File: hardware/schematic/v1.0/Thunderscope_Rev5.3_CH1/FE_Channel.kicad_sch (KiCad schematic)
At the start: 105 parts, among them J1002_1 BNC, K1000_1 G6K-2F-RF, K1001_1 G6K-2F-RF, Q1002_1 DMN62D0UW, Q1003_1 DMN62D0UW, U1001_1 TMUX4053, U1008_1 LMH6518, U1009_1 BUF802, U1011_1 OPA140AIDBVR

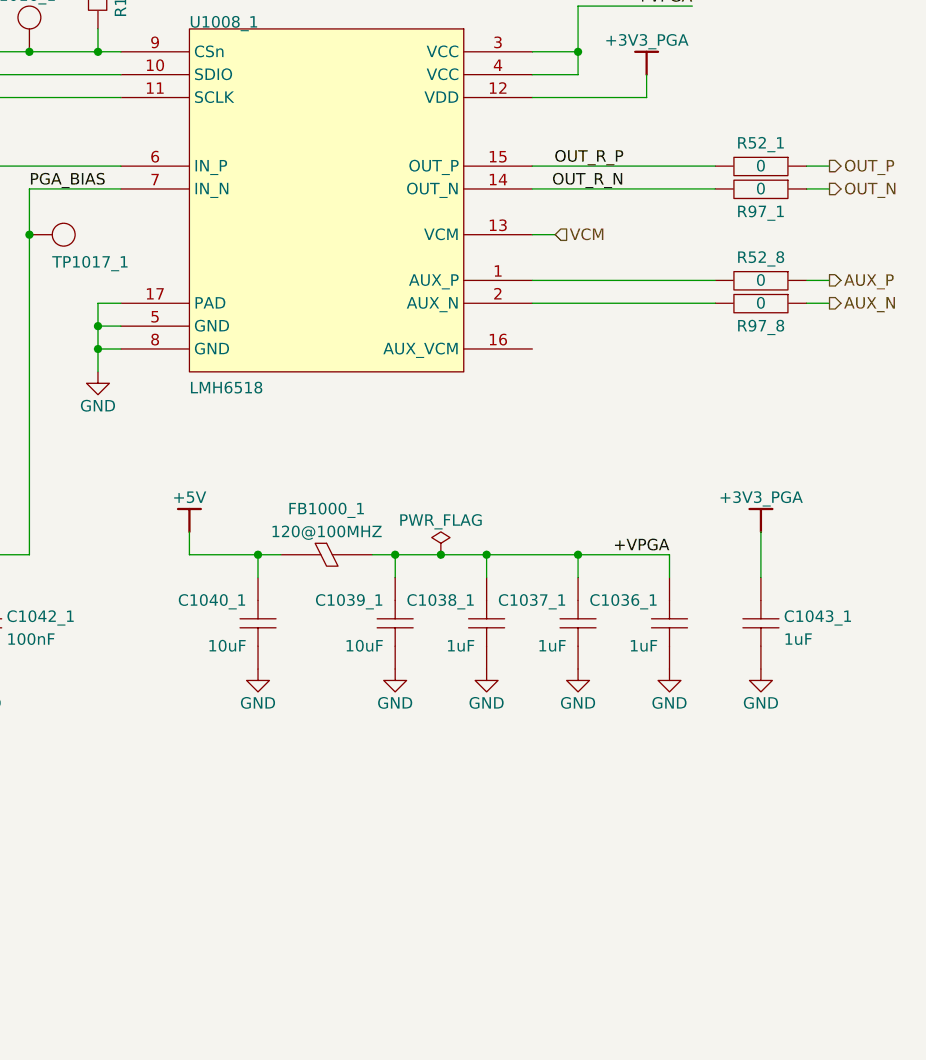
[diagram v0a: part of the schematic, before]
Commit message: sch and pcb update
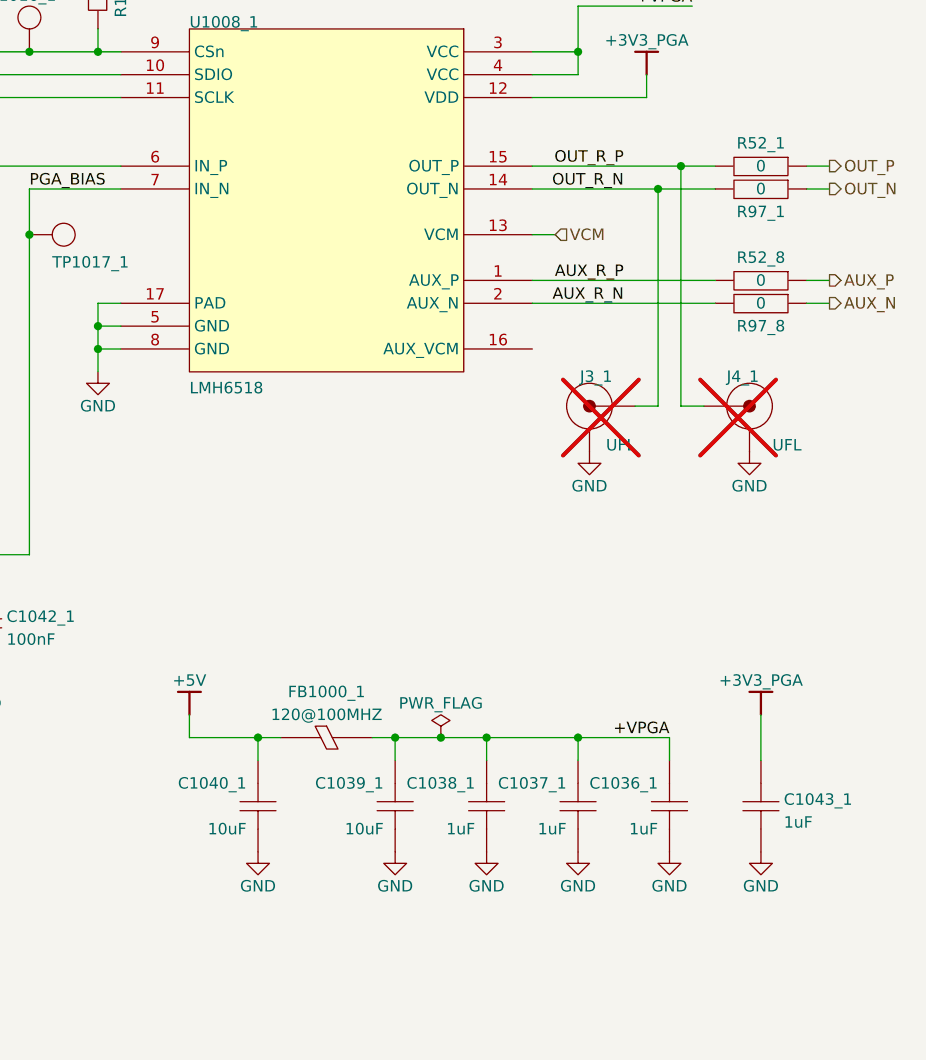
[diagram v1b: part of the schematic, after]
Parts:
- added J3_1, J4_1: UFL, Thunderscope_Rev5:TE_2334884-1, symbol Thunderscope_Rev5:UFL Jack SMD
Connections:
- net GND: now also J3_1.2 (SHIELD), J4_1.2 (SHIELD)
- net OUT_R_N: now also J3_1.1 (Signal)
- net OUT_R_P: now also J4_1.1 (Signal)
- net AUX_R_P: now reaches R52_8.1, U1008_1.1 (AUX_P)
- net AUX_R_N: now reaches R97_8.1, U1008_1.2 (AUX_N)
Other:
- moved on the sheet: C1036_1, C1037_1, C1038_1, C1039_1, C1040_1, C1043_1, FB1000_1

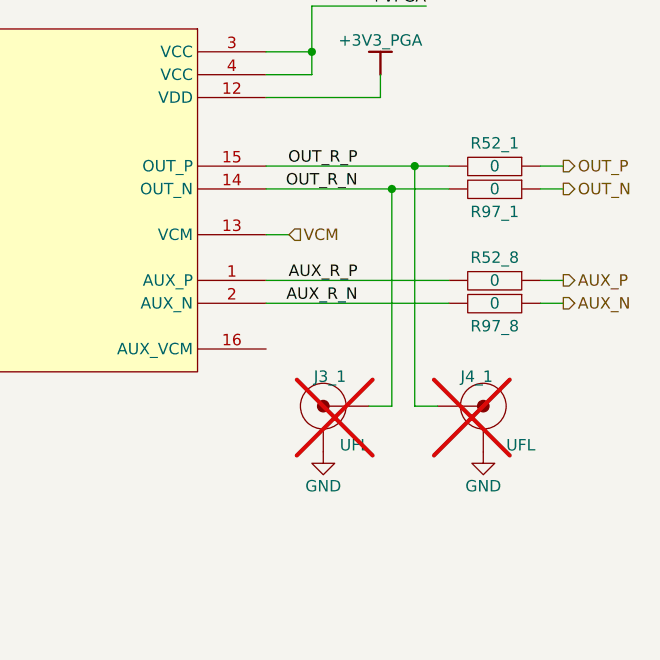
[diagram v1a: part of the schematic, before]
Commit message: sch and pcb update
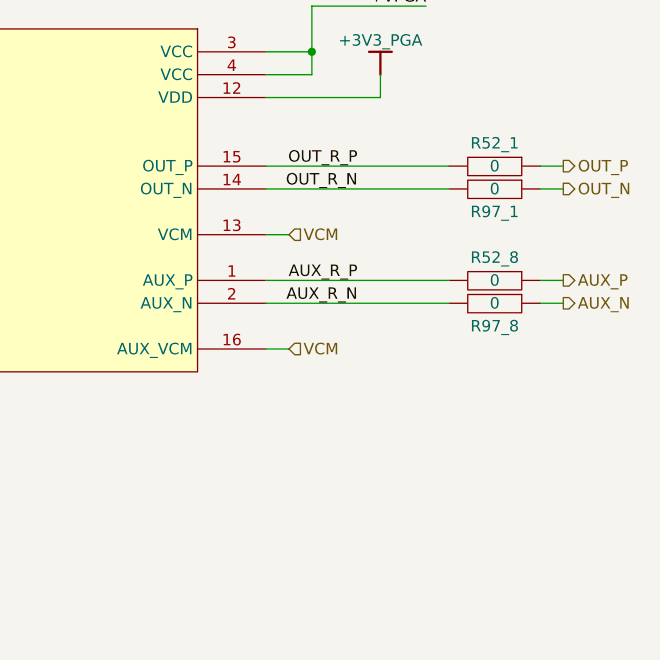
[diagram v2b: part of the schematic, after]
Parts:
- removed J3_1, J4_1: UFL, Thunderscope_Rev5:TE_2334884-1, symbol Thunderscope_Rev5:UFL Jack SMD
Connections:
- net VCM: now also U1008_1.16 (AUX_VCM)
